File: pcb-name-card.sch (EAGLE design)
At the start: 7 parts

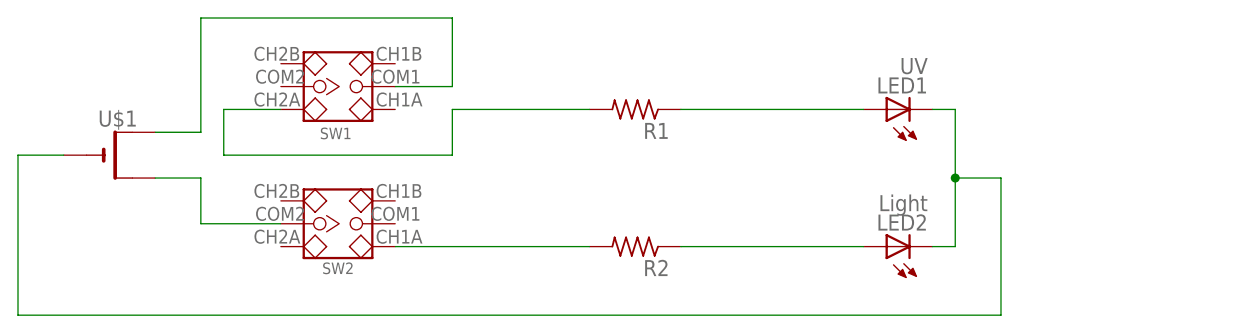
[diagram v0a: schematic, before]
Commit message: changes
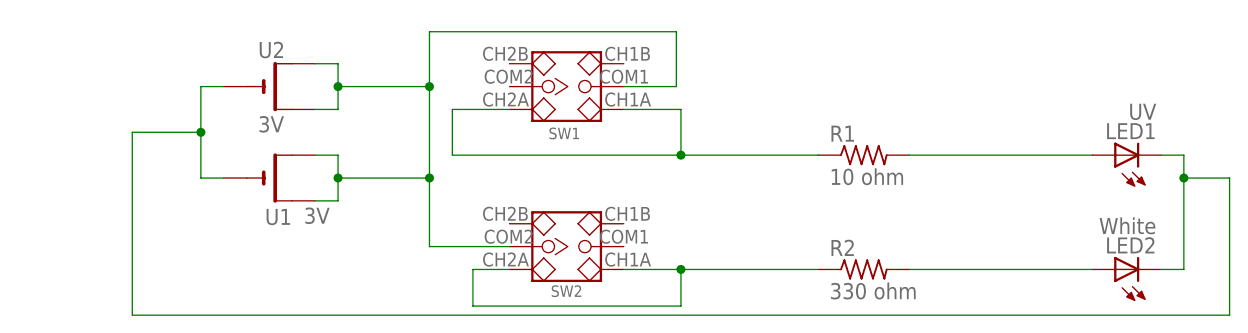
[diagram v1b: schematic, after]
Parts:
- removed U$1: (no value), cr2032:CR2032SMT
- added U1, U2: 3V, cr2032:CR2032SMT
- LED2: value Light -> White; device led:LEDCHIP-LED0805 -> led:LY_T679-D2E2-1
- R1: value (none) -> 10 ohm; device resistor:R-US_0207/7 -> resistor:R-US_R2010
- R2: value (none) -> 330 ohm; device resistor:R-US_0207/7 -> resistor:R-US_R2010
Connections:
- removed net N$3: SW1.COM1, U$1.+
- removed net N$6: LED1.C, LED2.C, U$1.-
- new net N$9: SW1.COM1, SW2.COM2, U1.+, U1.+1, U2.+, U2.+1
- net N$1: now also R1.2; no longer R1.1
- net N$2: now also R2.2; no longer R2.1
- net N$4: now also R1.1, SW1.CH1A; no longer R1.2
- net N$5: now also R2.1, SW2.CH2A; no longer R2.2
- net N$7: now also LED1.C, LED2.C, U1.-, U2.-; no longer SW2.COM2, U$1.+1
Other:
- moved on the sheet: LED1, LED2, R1, R2, SW1, SW2

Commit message: larger positive battery contacts
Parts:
- U1, U2: device cr2032:CR2032SMT -> cr2032-large-side:CR2032SMT
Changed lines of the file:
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@@
 <parts>
 <part name="LED1" library="led" deviceset="*_T679-?-1" device="D2E2" technology="LY" value="UV"/>
-<part name="U2" library="cr2032" deviceset="CR2032" device="SMT" value="3V"/>
+<part name="U2" library="cr2032-large-side" deviceset="CR2032" device="SMT" value="3V"/>
 <part name="SW1" library="Seeed-OPL-Switch" deviceset="SMD-TOGGLE-SWITCH-2CH(2X3P-7X3.5MM)" device=""/>
 <part name="SW2" library="Seeed-OPL-Switch" deviceset="SMD-TOGGLE-SWITCH-2CH(2X3P-7X3.5MM)" device=""/>
 <part name="LED2" library="led" deviceset="*_T679-?-1" device="D2E2" technology="LY" value="White"/>
-<part name="U1" library="cr2032" deviceset="CR2032" device="SMT" value="3V"/>
+<part name="U1" library="cr2032-large-side" deviceset="CR2032" device="SMT" value="3V"/>
 <part name="R1" library="resistor" deviceset="R-US_" device="R2010" value="10 ohm"/>
 <part name="R2" library="resistor" deviceset="R-US_" device="R2010" value="330 ohm"/>
